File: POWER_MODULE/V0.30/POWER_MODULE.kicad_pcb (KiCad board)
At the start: 2 copper layers, 88.1 x 113 mm, 100 parts, among them P1 CONN_8X2, Q1 IRLL3303, U1 TRACO-THN-15-1211, U2 L5973D

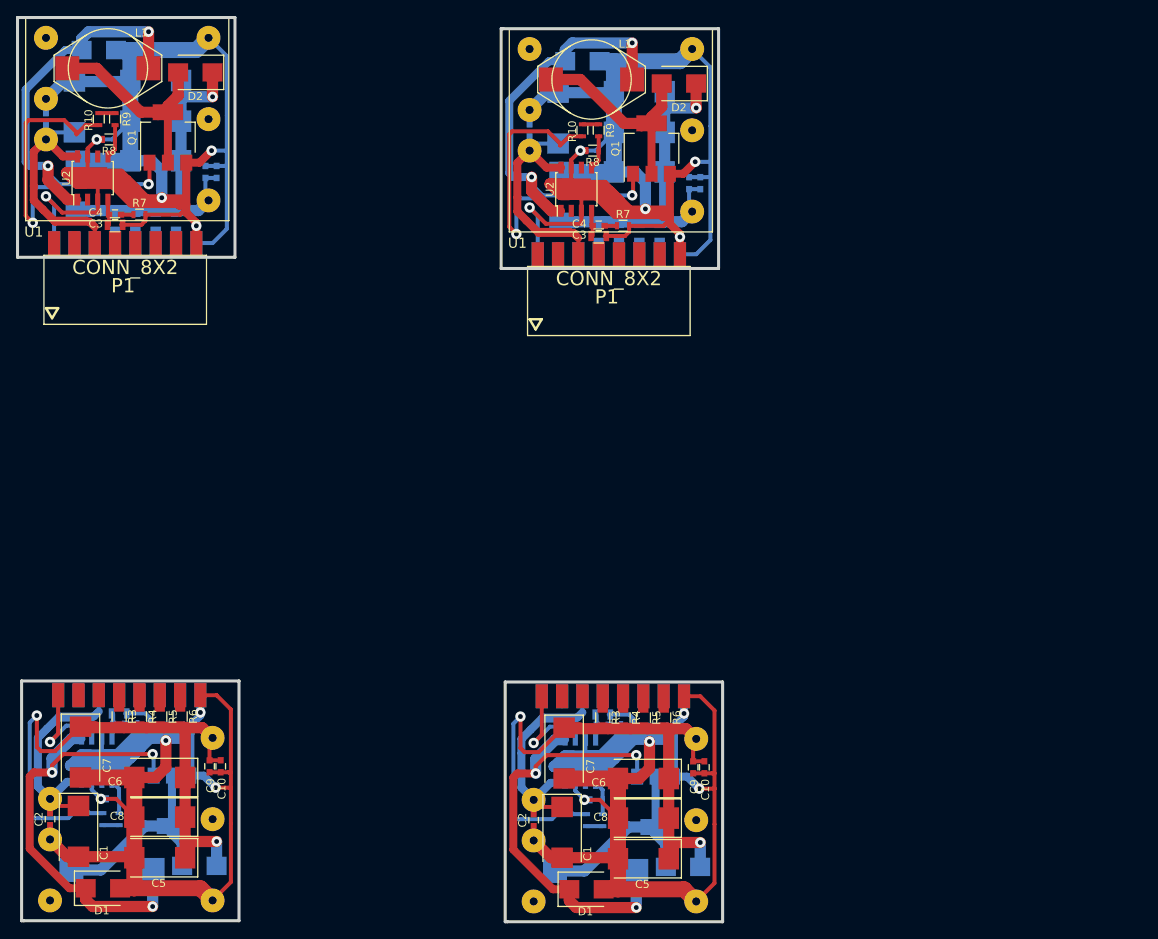
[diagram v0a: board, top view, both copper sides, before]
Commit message: MAJ
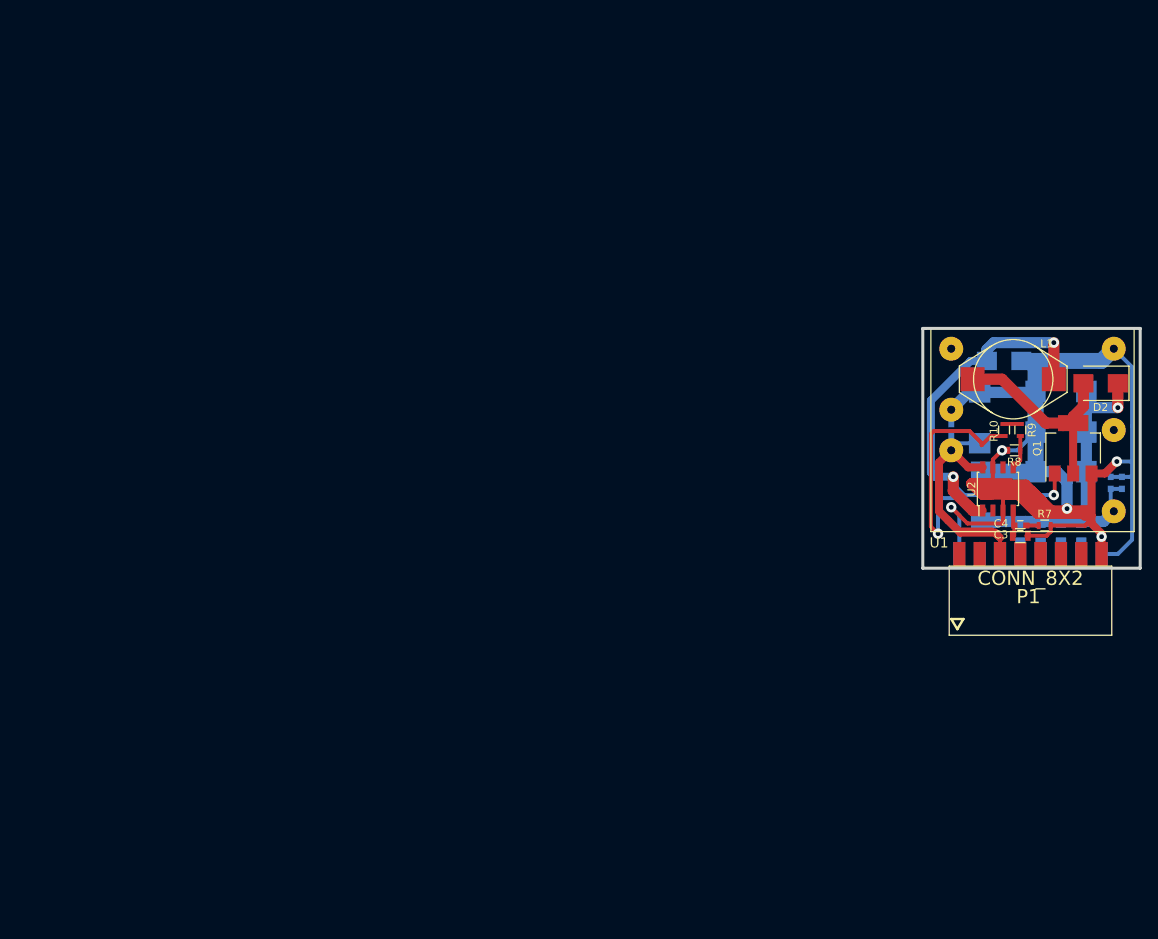
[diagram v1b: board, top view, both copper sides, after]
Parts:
- removed the C1 at (35.4, 149.5)
- removed the C1 at (95.9, 149.6)
- removed the C1 at (95.4, 60.3)
- removed the C10 at (53.2, 141.4)
- removed the C10 at (113.7, 141.5)
- removed the C10 at (113.2, 68.5)
- removed the C2 at (31.9, 148.0)
- removed the C2 at (92.3, 148.1)
- removed the C2 at (91.8, 61.8)
- removed the C3 at (40.5, 134.7)
- removed the C3 at (101.0, 134.9)
- removed the C3 at (100.5, 75.1)
- removed the C4 at (40.5, 136.0)
- removed the C4 at (101.0, 136.1)
- removed the C4 at (100.5, 73.8)
- removed the C5 at (45.6, 152.8)
- removed the C5 at (106.0, 152.9)
- removed the C5 at (105.5, 57.0)
- removed the C6 at (45.6, 142.7)
- removed the C6 at (106.0, 142.9)
- removed the C6 at (105.5, 67.1)
- removed the C7 at (35.7, 139.6)
- removed the C7 at (96.1, 139.7)
- removed the C7 at (95.6, 70.2)
- removed the C8 at (45.6, 147.7)
- removed the C8 at (106.0, 147.8)
- removed the C8 at (105.5, 62.1)
- removed the C9 at (51.8, 141.4)
- removed the C9 at (112.3, 141.5)
- removed the C9 at (111.8, 68.5)
- removed the D1 at (38.5, 156.6)
- removed the D1 at (98.9, 156.7)
- removed the D1 at (98.4, 53.2)
- removed the D2 at (50.5, 153.8)
- removed the D2 at (111.0, 153.9)
- removed the D2 at (110.5, 56.0)
- removed the L1 at (39.6, 154.3)
- removed the L1 at (100.1, 154.4)
- removed the L1 at (99.6, 55.5)
- removed the P1 at (50.7, 132.5)
- removed the P1 at (111.1, 132.6)
- removed the P1 at (110.6, 77.3)
- removed the Q1 at (47.1, 145.7)
- removed the Q1 at (107.6, 145.8)
- removed the Q1 at (107.1, 64.1)
- removed the R10 at (38.5, 148.0)
- removed the R10 at (98.9, 148.1)
- removed the R10 at (98.4, 61.8)
- removed the R3 at (40.5, 135.1)
- removed the R3 at (101.0, 135.3)
- removed the R3 at (100.5, 74.7)
- removed the R4 at (43.1, 135.1)
- removed the R4 at (103.5, 135.3)
- removed the R4 at (103.0, 74.7)
- removed the R5 at (45.6, 135.1)
- removed the R5 at (106.0, 135.3)
- removed the R5 at (105.5, 74.7)
- removed the R6 at (48.1, 135.1)
- removed the R6 at (108.6, 135.3)
- removed the R6 at (108.1, 74.7)
- removed the R7 at (43.6, 136.0)
- removed the R7 at (104.0, 136.1)
- removed the R7 at (103.5, 73.8)
- removed the R8 at (39.8, 145.4)
- removed the R8 at (100.2, 145.5)
- removed the R8 at (99.7, 64.4)
- removed the R9 at (40.5, 148.0)
- removed the R9 at (101.0, 148.1)
- removed the R9 at (100.5, 61.8)
- removed the U1 at (31.9, 158.1)
- removed the U1 at (92.3, 158.2)
- removed the U1 at (91.8, 51.7)
- removed the U2 at (37.7, 140.6)
- removed the U2 at (98.2, 140.7)
- removed the U2 at (97.7, 69.2)
- moved C2 119.6 mm to (144.5, 99.3)
- moved C3 119.6 mm to (153.2, 112.5)
- moved C4 119.6 mm to (153.2, 111.3)
- moved C7 119.6 mm to (148.3, 107.7)
- moved C9 119.6 mm to (164.5, 105.9)
- moved P1 119.6 mm to (163.3, 114.8)
- moved R3 119.6 mm to (153.2, 112.1)
- moved R6 119.6 mm to (160.8, 112.1)
- moved R7 119.6 mm to (156.2, 111.3)
- moved R8 119.6 mm to (152.4, 101.9)
- moved R9 119.6 mm to (153.2, 99.3)
- moved U1 119.6 mm to (144.5, 89.2)
- moved C1 119.6 mm to (148.1, 97.8)
- moved C10 119.6 mm to (165.9, 105.9)
- moved D1 119.6 mm to (151.1, 90.7)
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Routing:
- net GND: track 904.6 -> 226.1 mm, vias 20 -> 5
- net Net-(C10-Pad1): track 369.9 -> 92.5 mm, vias 8 -> 2
- net Net-(D1-Pad1): track 275.5 -> 68.9 mm, vias 12 -> 3
- net +BATT: track 185.8 -> 46.4 mm
- net Net-(D2-Pad2): track 112.4 -> 28.1 mm
- net Net-(R8-Pad1): track 17.1 -> 4.28 mm
- net Net-(C3-Pad1): track 12.8 -> 3.20 mm
- net Net-(R10-Pad2): track 8.13 -> 2.03 mm
- net +5VA: track 6.87 -> 1.72 mm
- net +5V: track 6.87 -> 1.72 mm
- net +3V3: track 6.87 -> 1.72 mm
- net +12V: track 6.87 -> 1.72 mm
- net Net-(C4-Pad2): track 6.19 -> 1.55 mm
- net /RA: track 4.06 -> 1.02 mm
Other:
- board size 88.1 x 113 mm -> 27.2 x 30 mm
